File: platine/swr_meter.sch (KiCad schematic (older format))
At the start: 25 parts, among them U1 CP0x0xx5425xNTR_Directional_C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, U2 LTC5530, U3 LM1117_SOT223, U4 STM32F030C8Tx, U5 STM32_mmvisual_JTAG, Y1 RESONATEUR

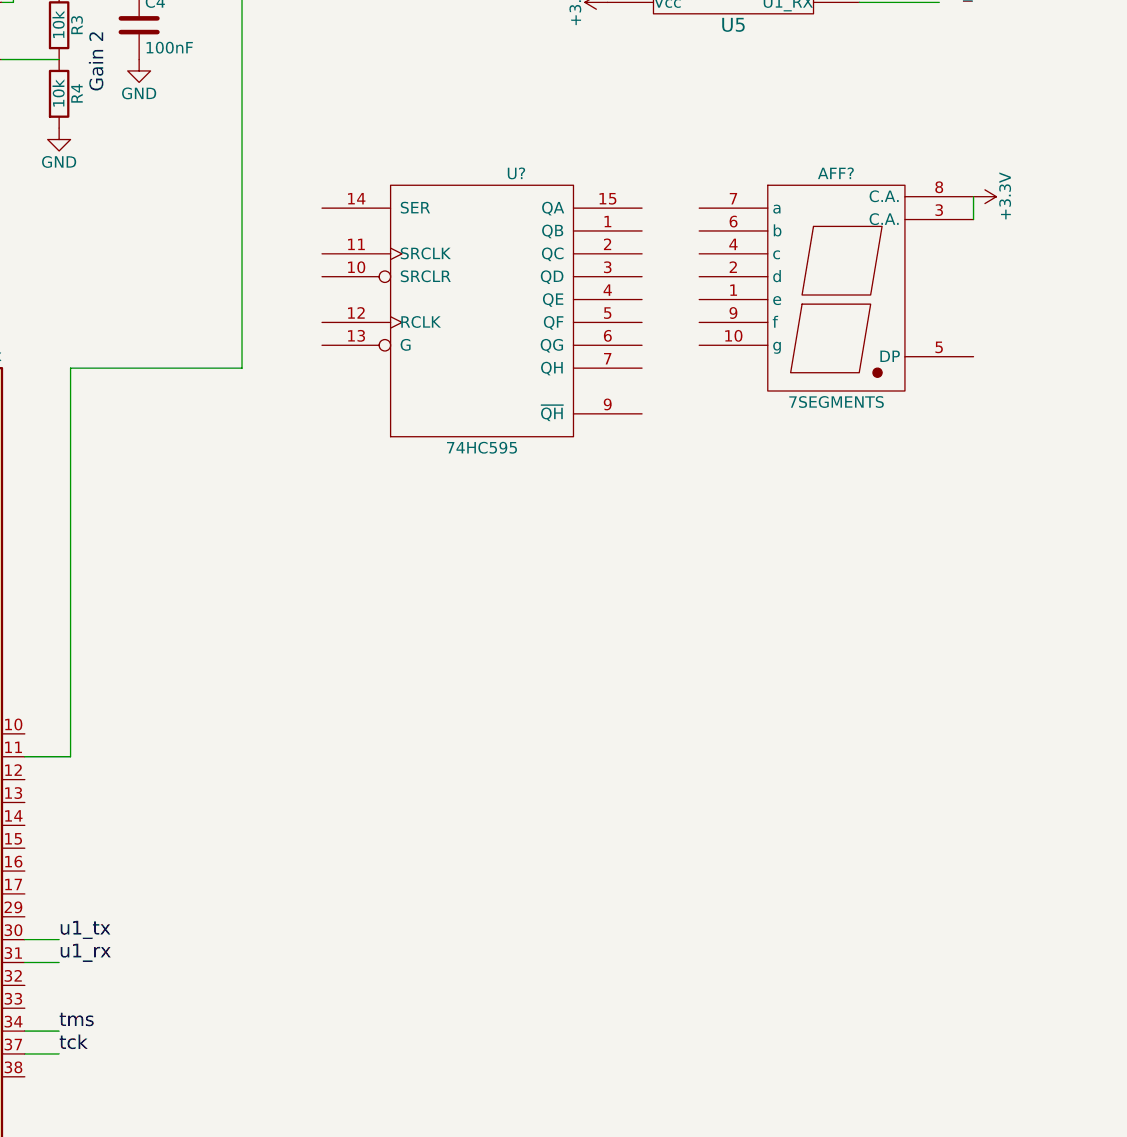
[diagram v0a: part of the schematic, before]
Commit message: work on 7-segment display
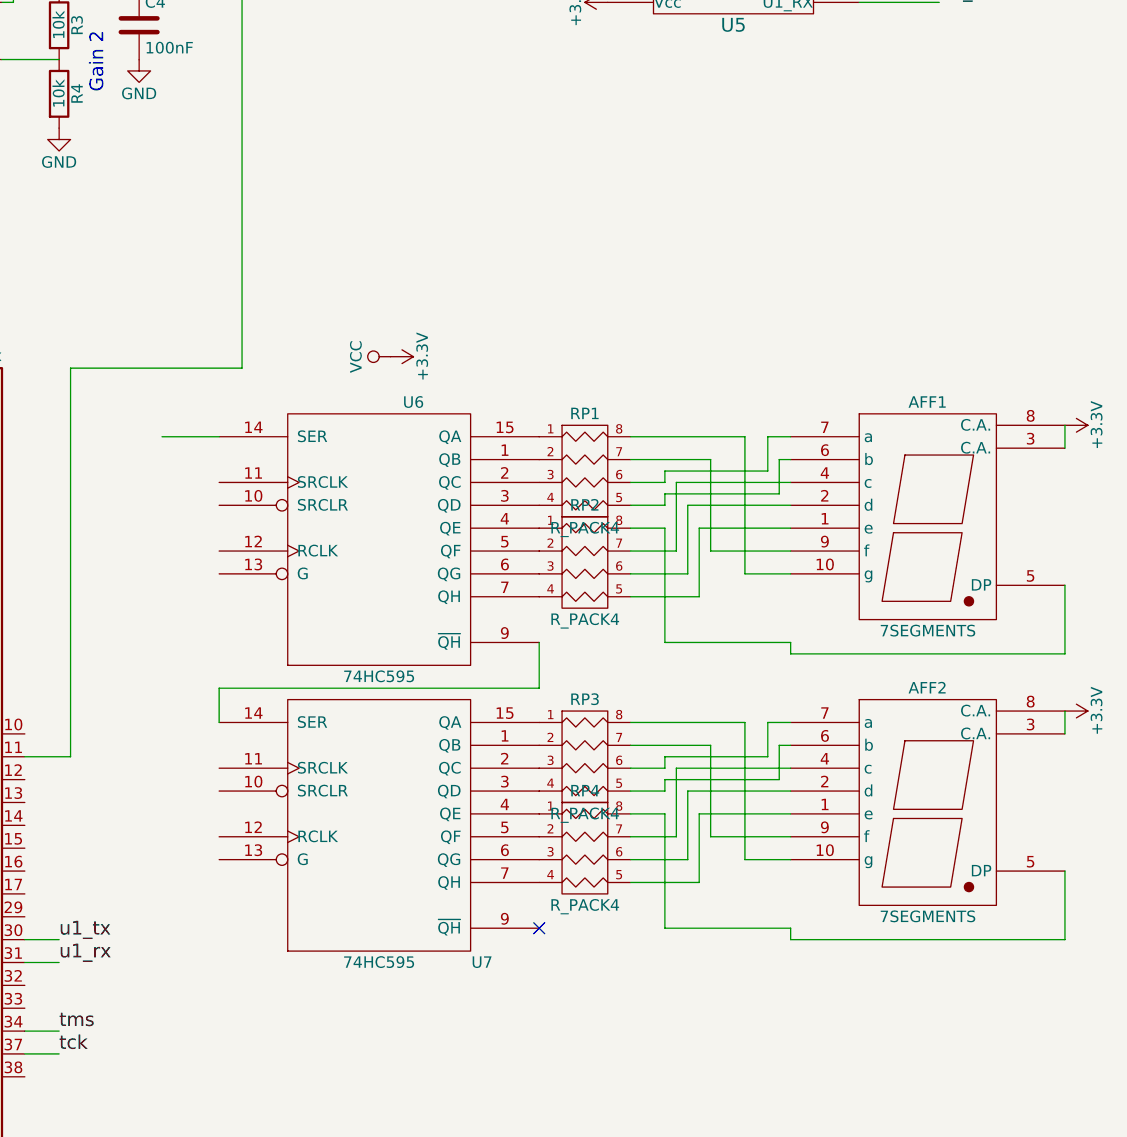
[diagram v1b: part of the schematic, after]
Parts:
- added AFF2: 7SEGMENTS, Housings_DIP:DIP-10_W7.62mm, symbol 7SEGMENTS
- added RP1, RP2, RP3, RP4: R_PACK4, Toni:R_array_4, symbol R_PACK4
- added U7: 74HC595, Housings_SOIC:SOIC-16_3.9x9.9mm_Pitch1.27mm, symbol 74HC595
- AFF1: renamed from AFF?; footprint (none) -> Housings_DIP:DIP-10_W7.62mm
- U6: renamed from U?; footprint (none) -> Housings_SOIC:SOIC-16_3.9x9.9mm_Pitch1.27mm
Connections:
- net VCC is gone; now on net +3V3: U6.16 (VCC)
- net +3V3: now also AFF2.3 (C.A.), AFF2.8 (C.A.), U7.16 (VCC)
- net GND: now also U7.8 (GND)
- net at AFF1.1 (e): now also RP2.5 (R4)
- net at AFF1.10 (g): now also RP1.8 (R1)
- net at AFF1.2 (d): now also RP2.6 (R3)
- net at AFF1.4 (c): now also RP2.7 (R2)
- net at AFF1.5 (DP): now also RP2.8 (R1)
- net at AFF1.6 (b): now also RP1.5 (R4)
- net at AFF1.7 (a): now also RP1.6 (R3)
- net at AFF1.9 (f): now also RP1.7 (R2)
- net at U6.1 (QB): now also RP1.2 (P2)
- net at U6.15 (QA): now also RP1.1 (P1)
- net at U6.2 (QC): now also RP1.3 (P3)
- net at U6.3 (QD): now also RP1.4 (P4)
- net at U6.4 (QE): now also RP2.1 (P1)
- net at U6.5 (QF): now also RP2.2 (P2)
- net at U6.6 (QG): now also RP2.3 (P3)
- net at U6.7 (QH): now also RP2.4 (P4)
- net at U6.9 (~QH): now also U7.14 (SER)
- new net: AFF2.1 (e), RP4.5 (R4)
- new net: AFF2.10 (g), RP3.8 (R1)
- new net: AFF2.2 (d), RP4.6 (R3)
- new net: AFF2.4 (c), RP4.7 (R2)
- new net: AFF2.5 (DP), RP4.8 (R1)
- new net: AFF2.6 (b), RP3.5 (R4)
- new net: AFF2.7 (a), RP3.6 (R3)
- new net: AFF2.9 (f), RP3.7 (R2)
- new net: RP3.2 (P2), U7.1 (QB)
- new net: RP3.1 (P1), U7.15 (QA)
- new net: RP3.3 (P3), U7.2 (QC)
- new net: RP3.4 (P4), U7.3 (QD)
- new net: RP4.1 (P1), U7.4 (QE)
- new net: RP4.2 (P2), U7.5 (QF)
- new net: RP4.3 (P3), U7.6 (QG)
- new net: RP4.4 (P4), U7.7 (QH)
- no-connect marks 3 -> 4
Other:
- moved on the sheet: AFF1, U6
